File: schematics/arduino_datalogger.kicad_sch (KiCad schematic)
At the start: 9 parts, among them J1 SD card module, J2 RTC module, SW1 SW_Push, U1 DHT22

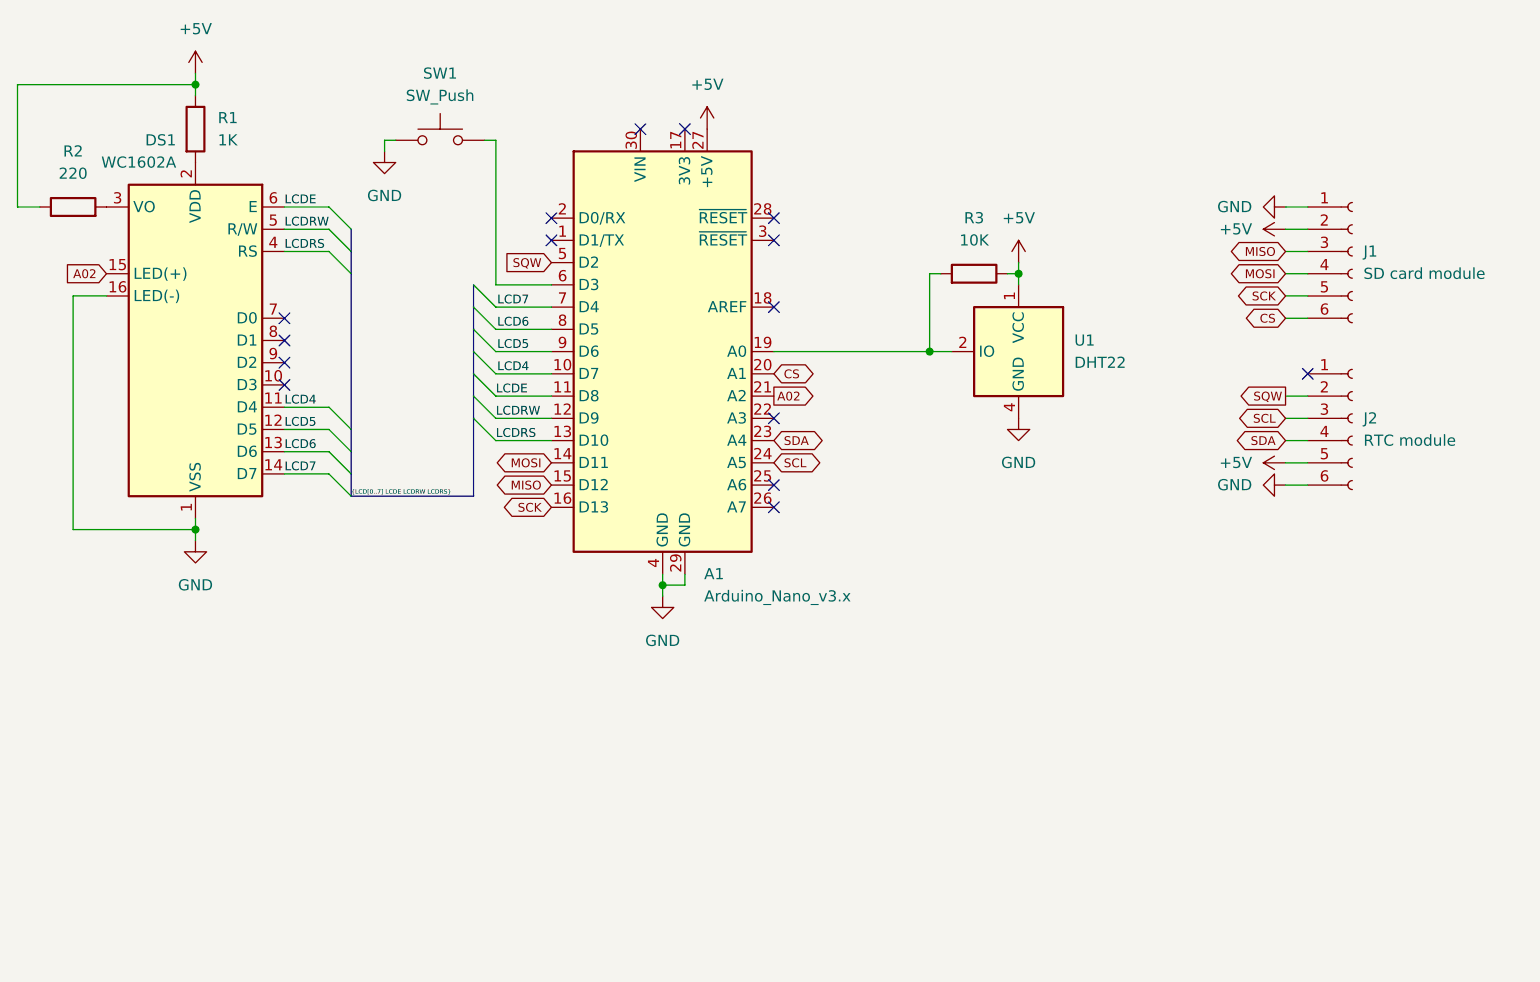
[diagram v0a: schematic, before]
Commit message: Algunos cambios esquema
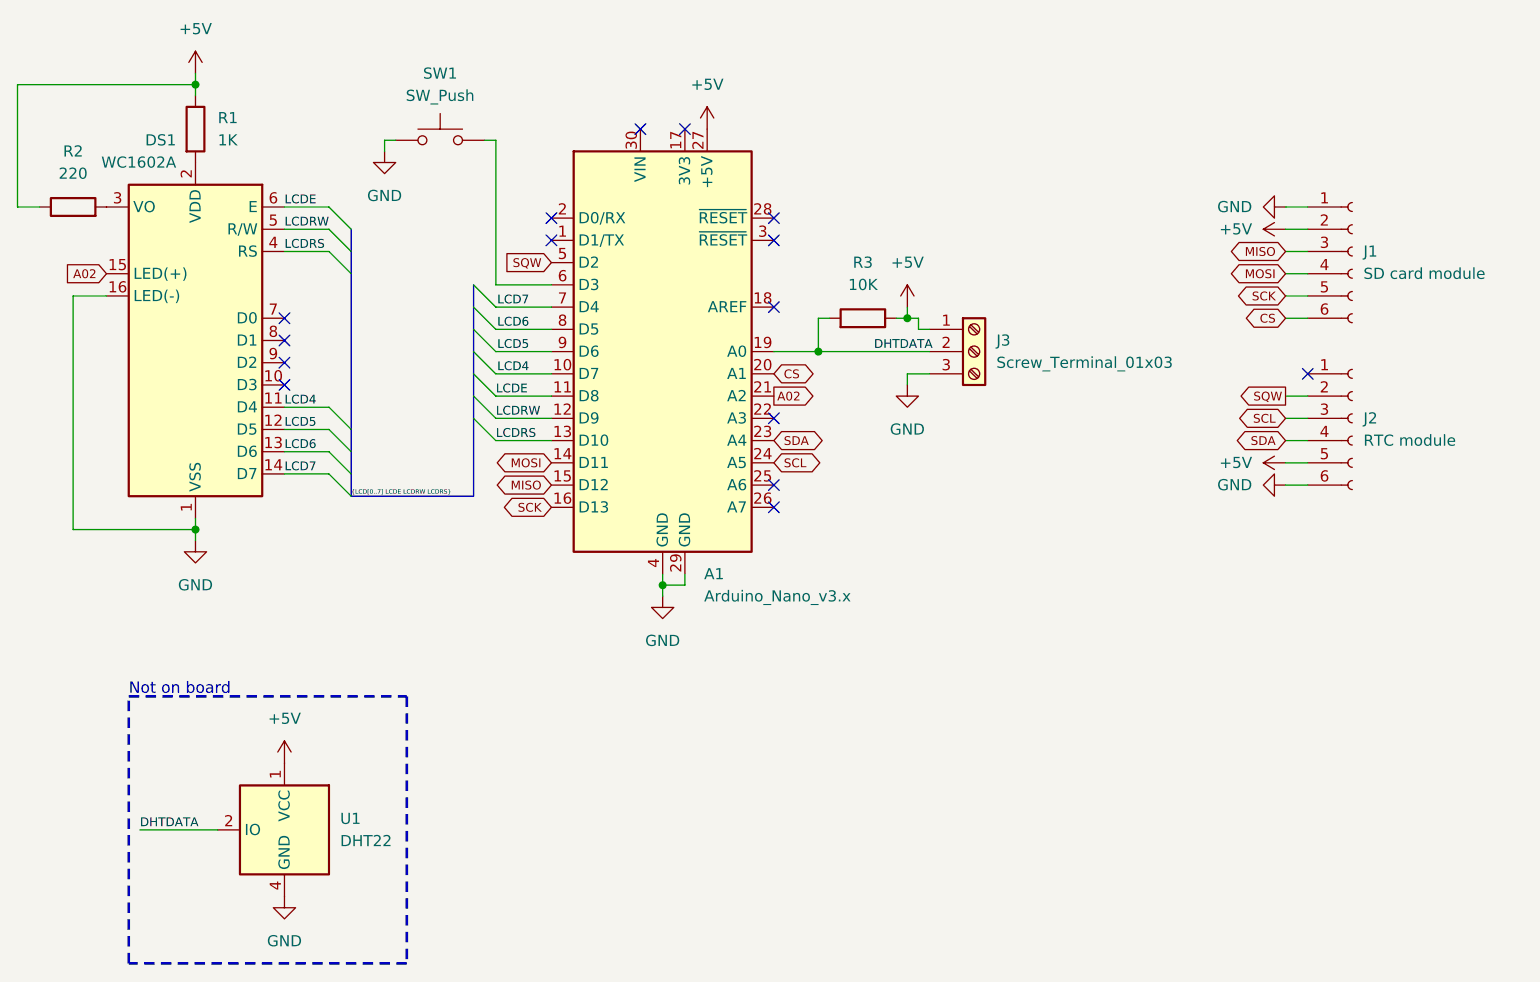
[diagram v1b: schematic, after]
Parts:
- added J3: Screw_Terminal_01x03, TerminalBlock:TerminalBlock_bornier-3_P5.08mm, symbol Connector:Screw_Terminal_01x03
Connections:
- net +5V: now also J3.1 (Pin_1)
- net GND: now also J3.3 (Pin_3)
- net DHTDATA: now reaches A1.19 (A0), R3.2, U1.2 (IO)
- net DHTDATA: now also J3.2 (Pin_2)
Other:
- note added: "Not on board"
- moved on the sheet: R3, U1
